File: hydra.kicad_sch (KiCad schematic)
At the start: 59 parts, among them J1 PC104 Interconnect, J2 STLINK/V2 Header, J3 STLINK/V2 Clone Header, J4 USB Conn, J5 UART Header, U2 AMS1117-3.3, U3 STM32F103VCTx, Y1 16mHz

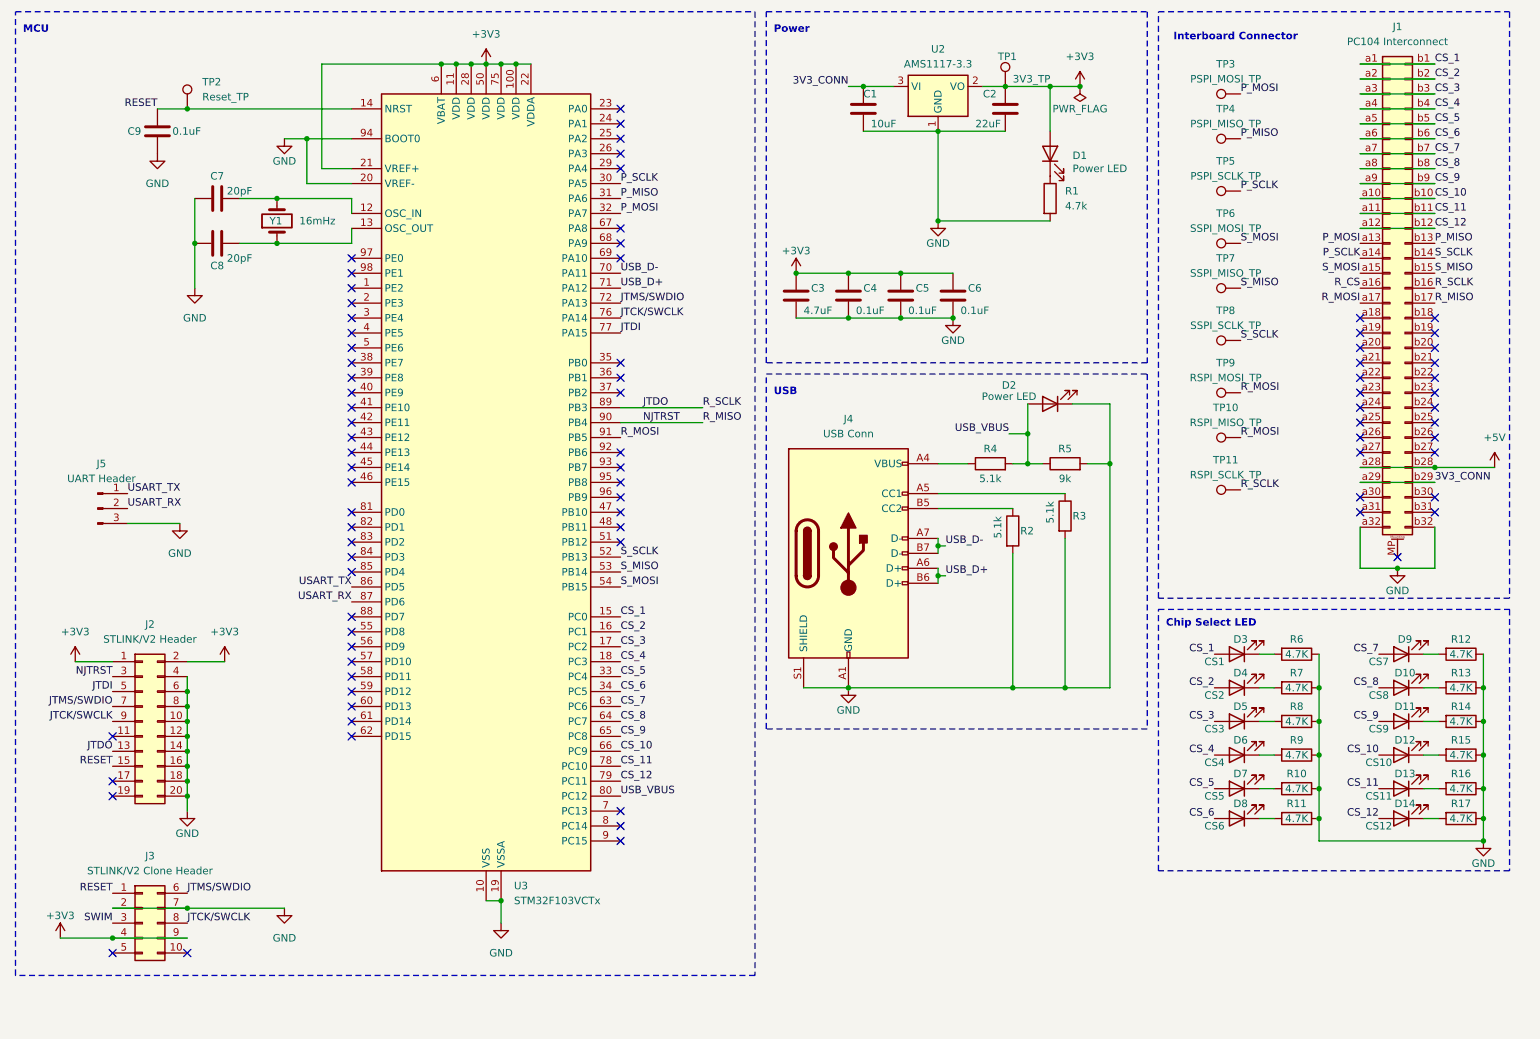
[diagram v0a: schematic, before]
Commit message: feat: mostly done pcb
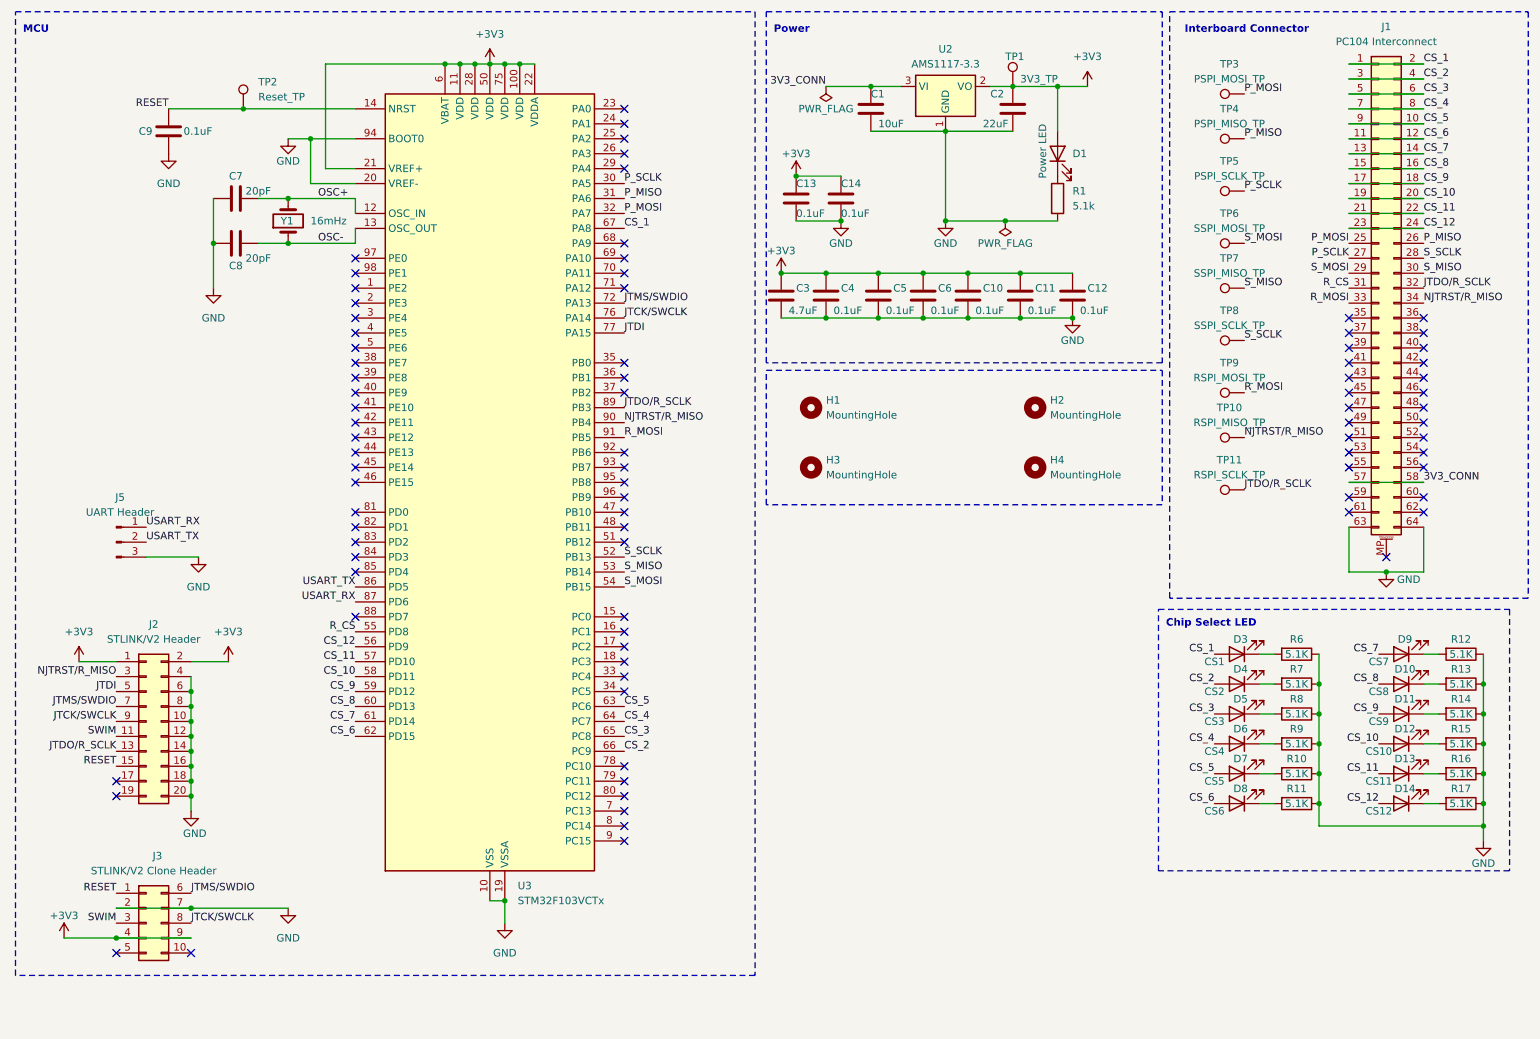
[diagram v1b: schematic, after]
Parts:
- removed D2: Power LED, symbol Device:LED
- removed J4: USB Conn, symbol Connector:USB_C_Receptacle_USB2.0_14P
- removed R2, R3, R4: 5.1k, symbol Device:R
- removed R5: 9k, symbol Device:R
- added C10, C11, C12, C13, C14: 0.1uF, Capacitor_SMD:C_0603_1608Metric, symbol Device:C
- added H1, H2, H3, H4: MountingHole, MountingHole:MountingHole_3.2mm_M3_DIN965_Pad, symbol Mechanical:MountingHole
- C1, C2, C3, C4, C5, C6, C7, C8, C9: footprint (none) -> Capacitor_SMD:C_0603_1608Metric
- D1, D10, D11, D12, D13, D14, D3, D4, D5, D6, D7, D8, D9: footprint (none) -> LED_SMD:LED_0603_1608Metric
- J1: footprint (none) -> Connector_PinHeader_2.54mm:PinHeader_2x32_P2.54mm_Vertical; symbol Connector_Generic_MountingPin:Conn_02x32_Row_Letter_First_MountingPin -> Connector_Generic_MountingPin:Conn_02x32_Odd_Even_MountingPin
- J2: footprint (none) -> Connector_PinHeader_2.54mm:PinHeader_2x10_P2.54mm_Vertical
- J3: footprint (none) -> Connector_PinHeader_2.54mm:PinHeader_2x05_P2.54mm_Vertical
- J5: footprint (none) -> Connector_PinHeader_2.54mm:PinHeader_1x03_P2.54mm_Vertical
- R1: value 4.7k -> 5.1k; footprint (none) -> Resistor_SMD:R_0603_1608Metric
- R10, R11, R12, R13, R14, R15, R16, R6, R7, R8, R9: value 4.7K -> 5.1K; footprint (none) -> Resistor_SMD:R_0603_1608Metric
- R17: value 4.7K -> 5.1K; footprint (none) -> Capacitor_SMD:C_0603_1608Metric
- TP1, TP10, TP11, TP2, TP3, TP4, TP5, TP6, TP7, TP8, TP9: footprint (none) -> TestPoint:TestPoint_Pad_D1.0mm
- Y1: footprint (none) -> Crystal:Crystal_HC49-U_Vertical
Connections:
- net +3V3: now also C10.1, C11.1, C12.1, C13.1, C14.1
- net 3V3_CONN: now also J1.57 (Pin_57), J1.58 (Pin_58); no longer J1.a29 (Pin_a29), J1.b29 (Pin_b29)
- net CS_1: now also J1.1 (Pin_1), J1.2 (Pin_2), U3.67 (PA8); no longer J1.a1 (Pin_a1), J1.b1 (Pin_b1), U3.15 (PC0)
- net CS_10: now also J1.19 (Pin_19), J1.20 (Pin_20), U3.58 (PD11); no longer J1.a10 (Pin_a10), J1.b10 (Pin_b10), U3.66 (PC9)
- net CS_11: now also J1.21 (Pin_21), J1.22 (Pin_22), U3.57 (PD10); no longer J1.a11 (Pin_a11), J1.b11 (Pin_b11), U3.78 (PC10)
- net CS_12: now also J1.23 (Pin_23), J1.24 (Pin_24), U3.56 (PD9); no longer J1.a12 (Pin_a12), J1.b12 (Pin_b12), U3.79 (PC11)
- net CS_2: now also J1.3 (Pin_3), J1.4 (Pin_4), U3.66 (PC9); no longer J1.a2 (Pin_a2), J1.b2 (Pin_b2), U3.16 (PC1)
- net CS_3: now also J1.5 (Pin_5), J1.6 (Pin_6), U3.65 (PC8); no longer J1.a3 (Pin_a3), J1.b3 (Pin_b3), U3.17 (PC2)
- net CS_4: now also J1.7 (Pin_7), J1.8 (Pin_8), U3.64 (PC7); no longer J1.a4 (Pin_a4), J1.b4 (Pin_b4), U3.18 (PC3)
- net CS_5: now also J1.10 (Pin_10), J1.9 (Pin_9), U3.63 (PC6); no longer J1.a5 (Pin_a5), J1.b5 (Pin_b5), U3.33 (PC4)
- net CS_6: now also J1.11 (Pin_11), J1.12 (Pin_12), U3.62 (PD15); no longer J1.a6 (Pin_a6), J1.b6 (Pin_b6), U3.34 (PC5)
- net CS_7: now also J1.13 (Pin_13), J1.14 (Pin_14), U3.61 (PD14); no longer J1.a7 (Pin_a7), J1.b7 (Pin_b7), U3.63 (PC6)
- net CS_8: now also J1.15 (Pin_15), J1.16 (Pin_16), U3.60 (PD13); no longer J1.a8 (Pin_a8), J1.b8 (Pin_b8), U3.64 (PC7)
- net CS_9: now also J1.17 (Pin_17), J1.18 (Pin_18), U3.59 (PD12); no longer J1.a9 (Pin_a9), J1.b9 (Pin_b9), U3.65 (PC8)
- net GND: now also J1.63 (Pin_63), J1.64 (Pin_64), C10.2, C11.2, C12.2, C13.2, C14.2; no longer J1.a32 (Pin_a32), J1.b32 (Pin_b32)
- net P_MISO: now also J1.26 (Pin_26); no longer J1.b13 (Pin_b13)
- net P_MOSI: now also J1.25 (Pin_25); no longer J1.a13 (Pin_a13)
- net P_SCLK: now also J1.27 (Pin_27); no longer J1.a14 (Pin_a14)
- net R_CS: now also J1.31 (Pin_31), U3.55 (PD8); no longer J1.a16 (Pin_a16)
- net R_MOSI: now also J1.33 (Pin_33); no longer J1.a17 (Pin_a17), TP10.1
- net SWIM: now also J2.11 (Pin_11)
- net S_MISO: now also J1.30 (Pin_30); no longer J1.b15 (Pin_b15)
- net S_MOSI: now also J1.29 (Pin_29); no longer J1.a15 (Pin_a15)
- net S_SCLK: now also J1.28 (Pin_28); no longer J1.b14 (Pin_b14)
- net USART_RX: now also J5.1 (Pin_1); no longer J5.2 (Pin_2)
- net USART_TX: now also J5.2 (Pin_2); no longer J5.1 (Pin_1)
- net OSC-: now reaches C8.2, U3.13 (OSC_OUT), Y1.1
- net OSC+: now reaches C7.2, U3.12 (OSC_IN), Y1.2
- removed net +5V: J1.a28 (Pin_a28), J1.b28 (Pin_b28)
- net JTDO renamed JTDO/R_SCLK
- net JTDO/R_SCLK: now also J1.32 (Pin_32); no longer J1.b16 (Pin_b16)
- net NJTRST renamed NJTRST/R_MISO
- net NJTRST/R_MISO: now also J1.34 (Pin_34), TP10.1; no longer J1.b17 (Pin_b17)
- net USB_D+: no longer names the net of U3.71 (PA12)
- net USB_D-: no longer names the net of U3.70 (PA11)
- net USB_VBUS: no longer names the net of U3.80 (PC12)
- no-connect marks 81 -> 84
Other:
- note removed: "USB"
- moved on the sheet: C1, C2, C3, C4, C5, C6, C7, C8, C9, D1, D10, D11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

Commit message: feat: trying multinodal
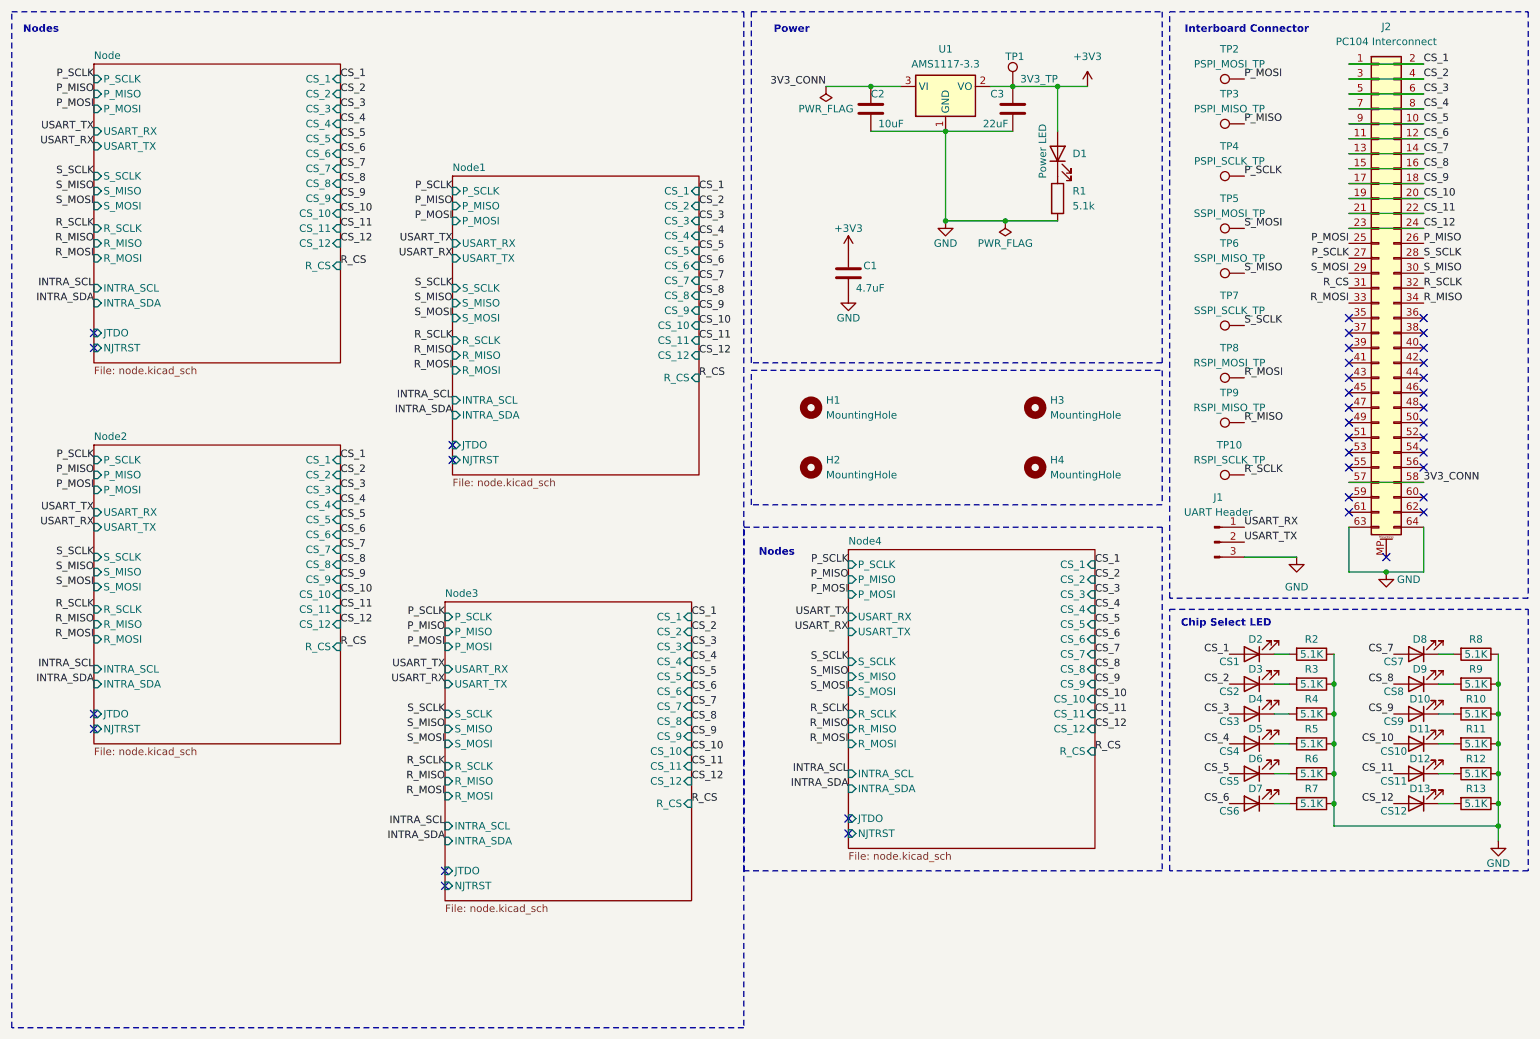
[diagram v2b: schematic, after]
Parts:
- removed C10, C11, C12, C13, C14, C4, C5, C6, C9: 0.1uF, Capacitor_SMD:C_0603_1608Metric, symbol Device:C
- removed C7, C8: 20pF, Capacitor_SMD:C_0603_1608Metric, symbol Device:C
- removed J2: STLINK/V2 Header, Connector_PinHeader_2.54mm:PinHeader_2x10_P2.54mm_Vertical, symbol Connector_Generic:Conn_02x10_Odd_Even
- removed J3: STLINK/V2 Clone Header, Connector_PinHeader_2.54mm:PinHeader_2x05_P2.54mm_Vertical, symbol Connector_Generic:Conn_02x05_Top_Bottom
- removed J5: UART Header, Connector_PinHeader_2.54mm:PinHeader_1x03_P2.54mm_Vertical, symbol Connector:Conn_01x03_Pin
- removed TP2: Reset_TP, TestPoint:TestPoint_Pad_D1.0mm, symbol Connector:TestPoint
- removed U3: STM32F103VCTx, Package_QFP:LQFP-100_14x14mm_P0.5mm, symbol MCU_ST_STM32F1:STM32F103VCTx
- removed Y1: 16mHz, Crystal:Crystal_HC49-U_Vertical, symbol Device:Crystal
- added J1: UART Header, Connector_PinHeader_2.54mm:PinHeader_1x03_P2.54mm_Vertical, symbol Connector:Conn_01x03_Pin
- renumbered C3 to C1, C1 to C2, C2 to C3, D11 to D10, D12 to D11, D13 to D12, D14 to D13, D3 to D2, D4 to D3, D5 to D4, D6 to D5, D7 to D6, D8 to D7, D9 to D8, D10 to D9, H3 to H2, H2 to H3, J1 to J2, R14 to R10, R15 to R11, R16 to R12, R17 to R13, R6 to R2, R7 to R3, R8 to R4, R9 to R5, R10 to R6, R11 to R7, R12 to R8, R13 to R9, TP11 to TP10, TP3 to TP2, TP4 to TP3, TP5 to TP4, TP6 to TP5, TP7 to TP6, TP8 to TP7, TP9 to TP8, TP10 to TP9, U2 to U1
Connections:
- net GND: now also J1.3 (Pin_3)
- net USART_RX: now also J1.1 (Pin_1)
- net USART_TX: now also J1.2 (Pin_2)
- net JTDO/R_SCLK renamed R_SCLK
- net NJTRST/R_MISO renamed R_MISO
- no-connect marks 84 -> 37
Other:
- added sheet Node (node.kicad_sch)
- added sheet Node1 (node.kicad_sch)
- added sheet Node2 (node.kicad_sch)
- added sheet Node3 (node.kicad_sch)
- added sheet Node4 (node.kicad_sch)
- note added: "Nodes"
- note removed: "MCU"
- moved on the sheet: C1, D10, D11, D12, D13, D2, D3, D4, D5, D6, D7, D8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

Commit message: feat: in progress rework
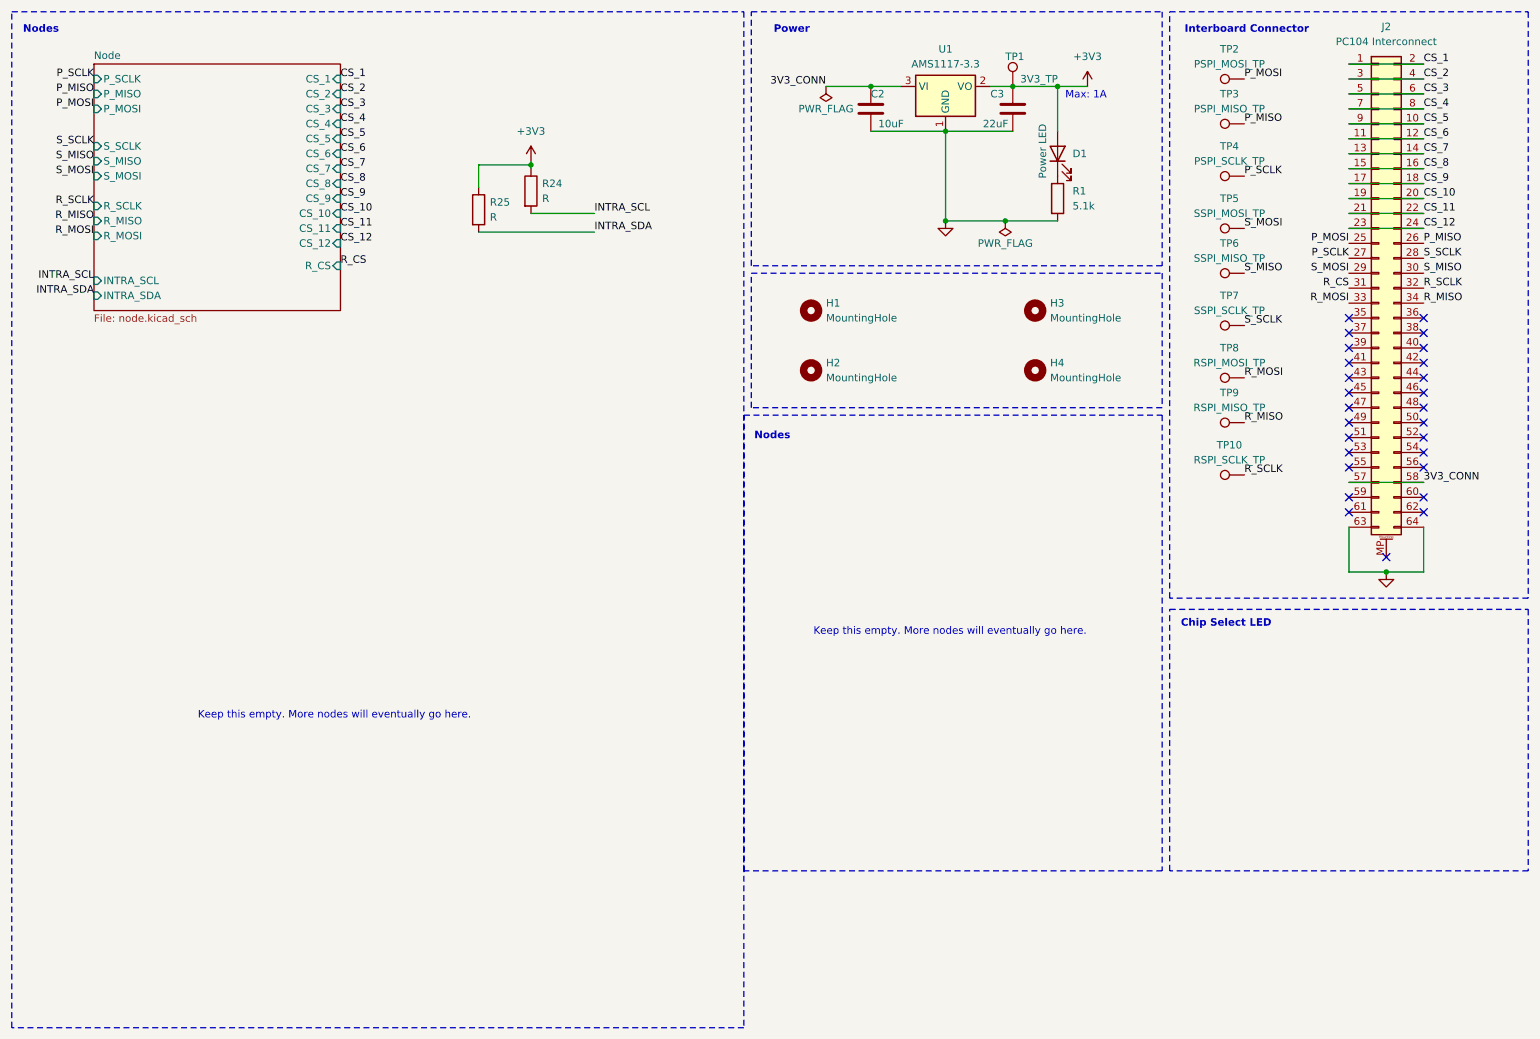
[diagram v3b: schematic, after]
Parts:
- removed C1: 4.7uF, Capacitor_SMD:C_0603_1608Metric, symbol Device:C
- removed D10: CS9, LED_SMD:LED_0603_1608Metric, symbol Device:LED
- removed D11: CS10, LED_SMD:LED_0603_1608Metric, symbol Device:LED
- removed D12: CS11, LED_SMD:LED_0603_1608Metric, symbol Device:LED
- removed D13: CS12, LED_SMD:LED_0603_1608Metric, symbol Device:LED
- removed D2: CS1, LED_SMD:LED_0603_1608Metric, symbol Device:LED
- removed D3: CS2, LED_SMD:LED_0603_1608Metric, symbol Device:LED
- removed D4: CS3, LED_SMD:LED_0603_1608Metric, symbol Device:LED
- removed D5: CS4, LED_SMD:LED_0603_1608Metric, symbol Device:LED
- removed D6: CS5, LED_SMD:LED_0603_1608Metric, symbol Device:LED
- removed D7: CS6, LED_SMD:LED_0603_1608Metric, symbol Device:LED
- removed D8: CS7, LED_SMD:LED_0603_1608Metric, symbol Device:LED
- removed D9: CS8, LED_SMD:LED_0603_1608Metric, symbol Device:LED
- removed J1: UART Header, Connector_PinHeader_2.54mm:PinHeader_1x03_P2.54mm_Vertical, symbol Connector:Conn_01x03_Pin
- removed R10, R11, R12, R2, R3, R4, R5, R6, R7, R8, R9: 5.1K, Resistor_SMD:R_0603_1608Metric, symbol Device:R
- removed R13: 5.1K, Capacitor_SMD:C_0603_1608Metric, symbol Device:R
- added R24, R25: R, symbol Device:R
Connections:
- net +3V3: now also R24.1, R25.1
- net INTRA_SCL: now also R24.2
- net INTRA_SDA: now also R25.2
- no-connect marks 37 -> 27
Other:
- removed sheet Node1
- removed sheet Node2
- removed sheet Node3
- removed sheet Node4
- sheet Node ports: added none; removed JTDO, NJTRST, USART_RX, USART_TX
- note added: "Keep this empty. More nodes will eventually go here."
- note added: "Max: 1A"
- moved on the sheet: H1, H2, H3, H4
